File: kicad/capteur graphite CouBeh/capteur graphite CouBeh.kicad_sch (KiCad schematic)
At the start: 19 parts, among them J1 Power, J2 Digital/PWM, J3 Analog, J4 Digital/PWM, J5 Conn_01x02, U2 LTC1050, U3 MCP41050

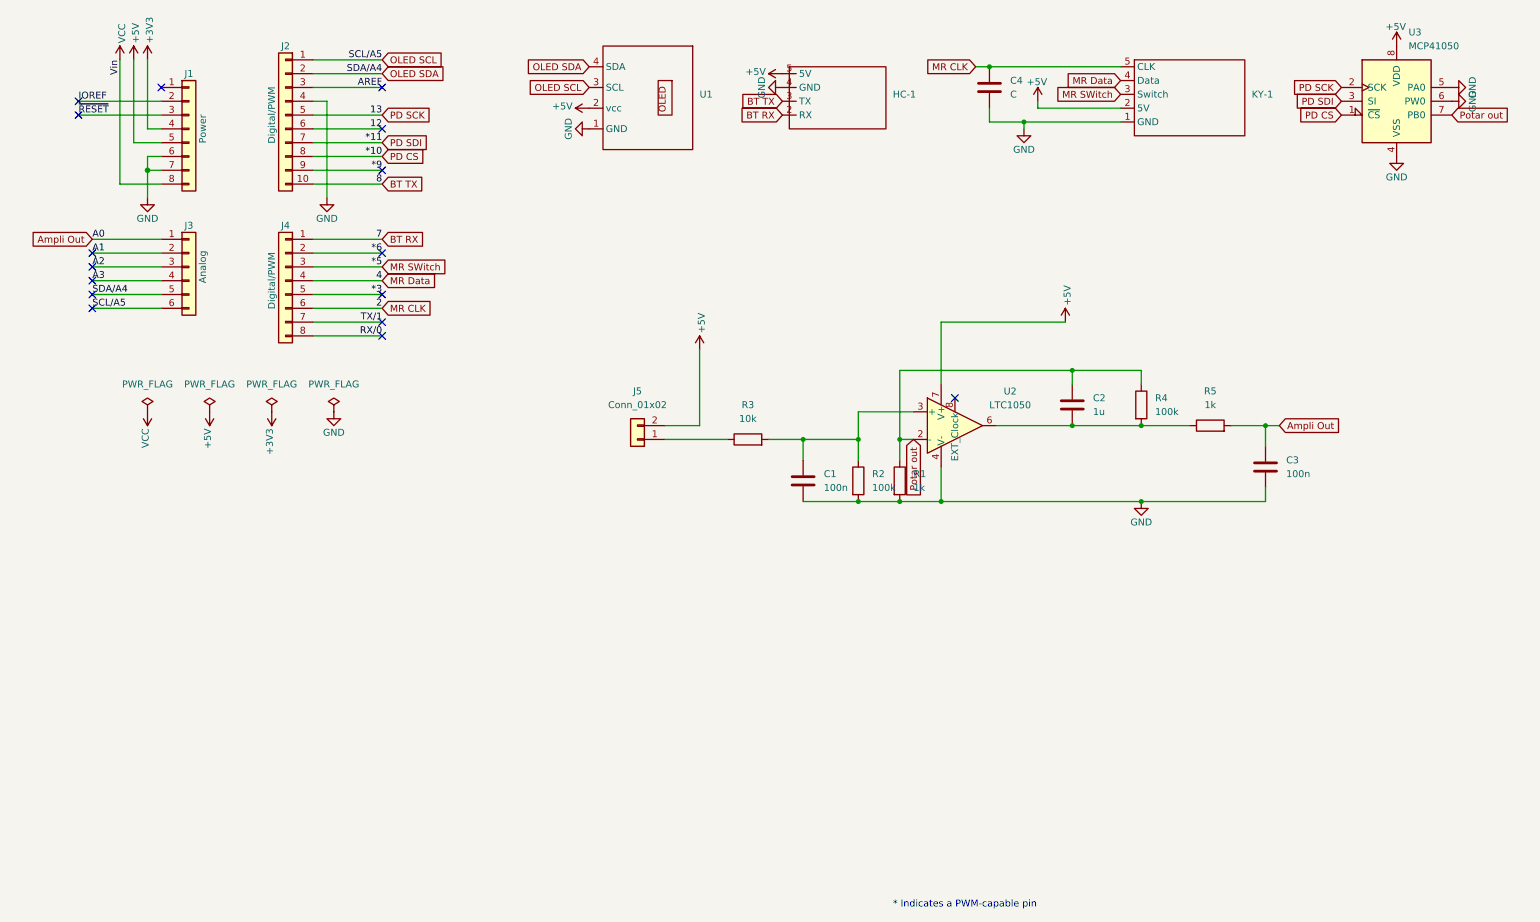
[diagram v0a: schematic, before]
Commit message: Add files via upload
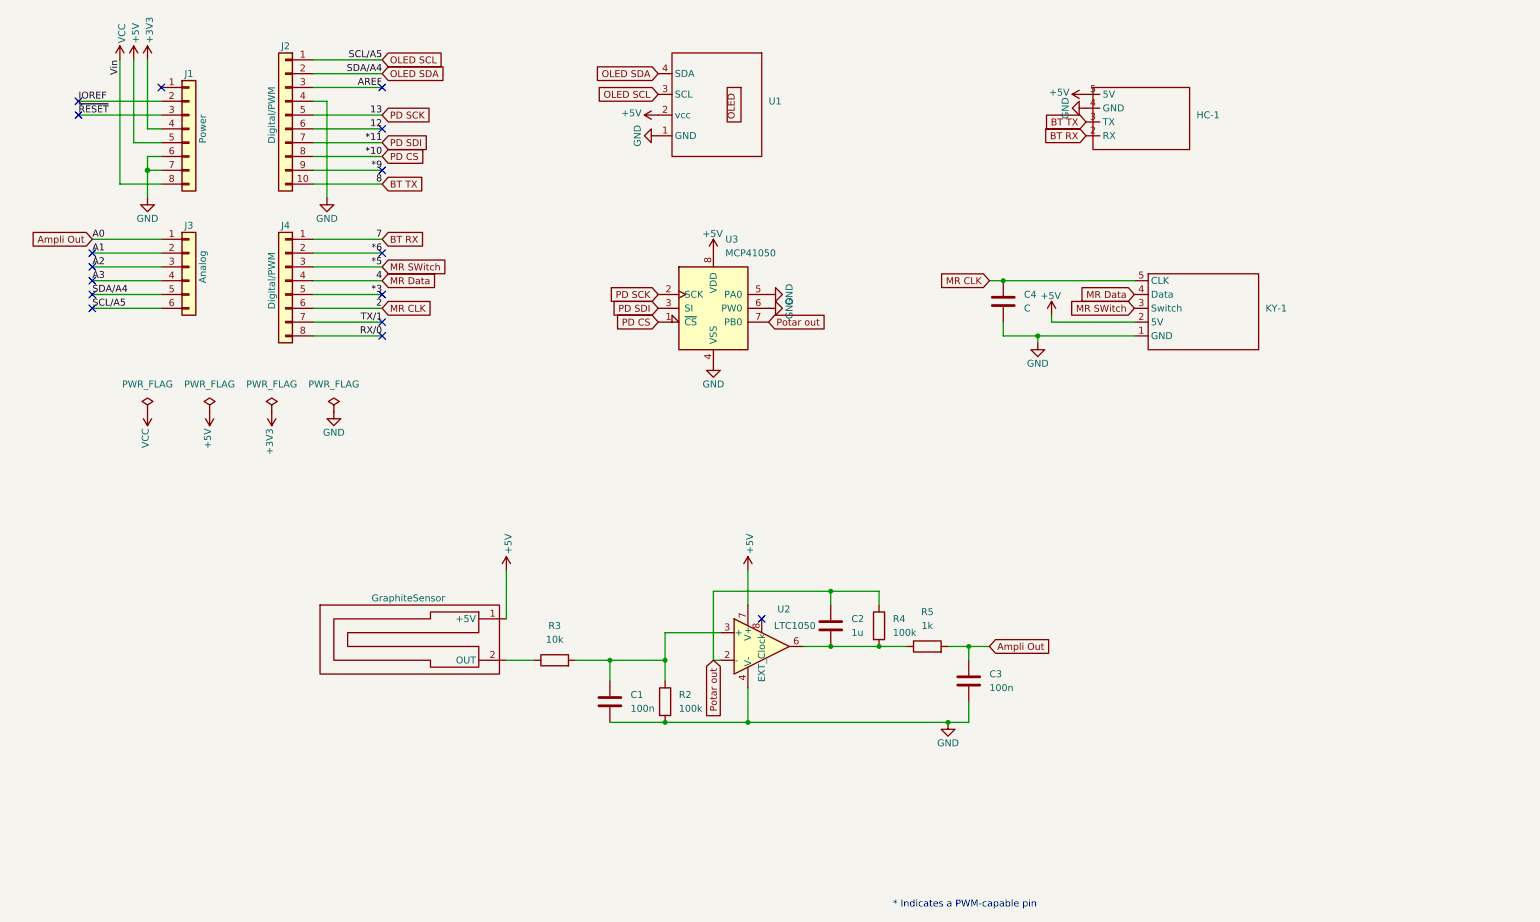
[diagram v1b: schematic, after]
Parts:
- removed J5: Conn_01x02, Connector_PinSocket_2.54mm:PinSocket_1x02_P2.54mm_Vertical, symbol Connector_Generic:Conn_01x02
- removed R1: 1k, Resistor_THT:R_Axial_DIN0204_L3.6mm_D1.6mm_P7.62mm_Horizontal, symbol Device:R
- added GraphiteSensor: ~, symbol ma lib graphite coubeh:Graphite_Sensor
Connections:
- net +5V: now also GraphiteSensor.1 (+5V)
- net at R3.1: now also GraphiteSensor.2 (OUT)
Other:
- moved on the sheet: C1, C2, C3, C4, HC-1, KY-1, R2, R3, R4, R5, U1, U2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
